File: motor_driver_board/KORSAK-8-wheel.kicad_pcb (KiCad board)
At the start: 2 copper layers, 170 x 90 mm, 20 parts, among them J1 Screw_Terminal_01x04, J2 Conn_01x02_Male, J3 Screw_Terminal_01x06, J4 Screw_Terminal_01x04, M1 Motor_DC, M2 Motor_DC, M3 Motor_DC, M4 Motor_DC, M5 Motor_DC, M6 Motor_DC, M7 Motor_DC, M8 Motor_DC, U1 L293D, U2 L293D, U3 L293D, U4 L293D

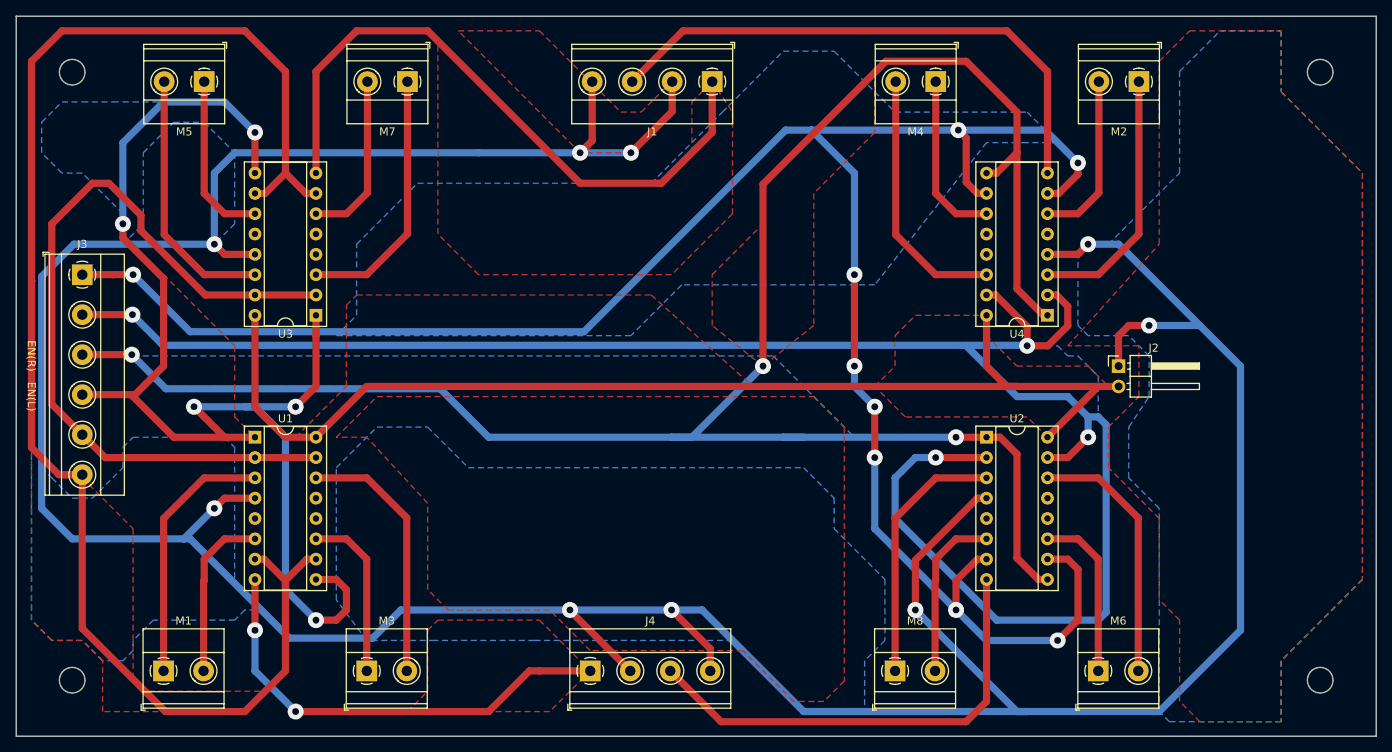
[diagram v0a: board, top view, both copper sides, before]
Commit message: Закончил моделировать плату
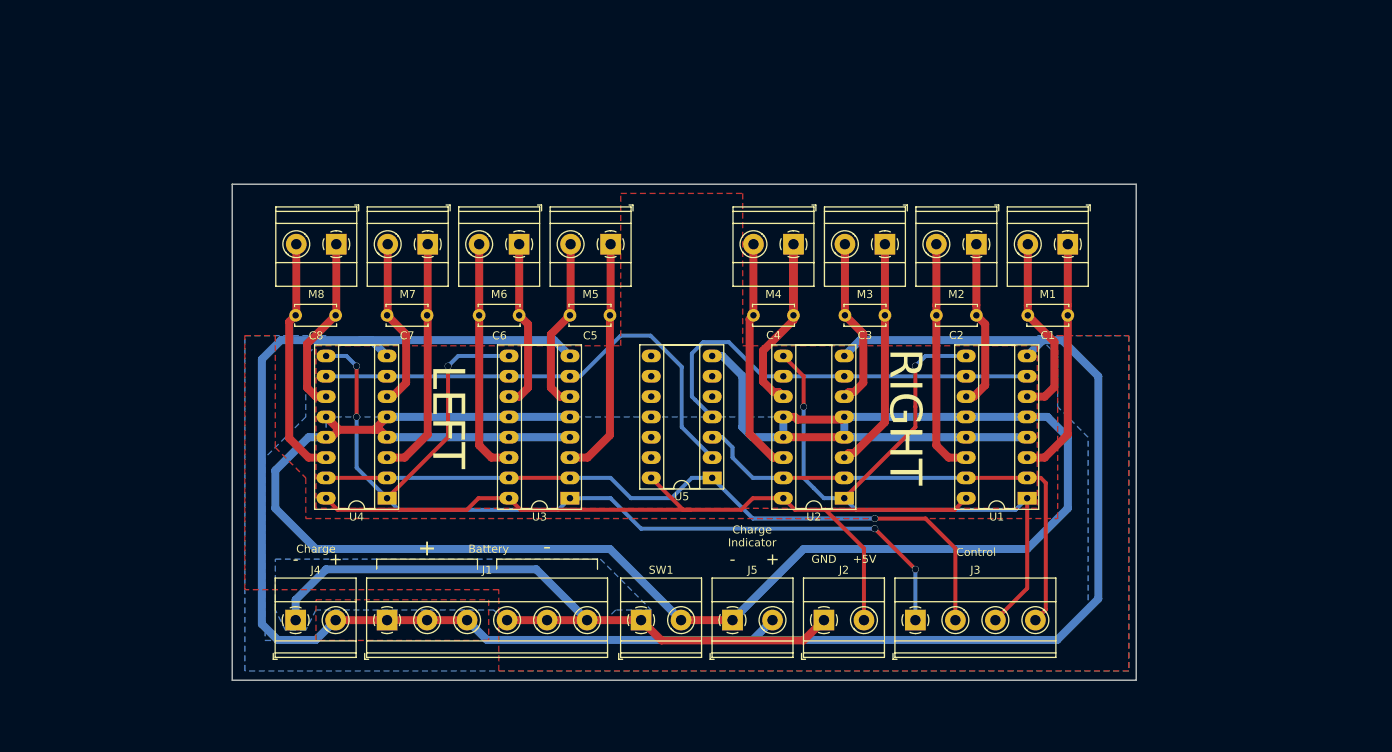
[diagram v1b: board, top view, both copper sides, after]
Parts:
- removed  : MountingHole_3.2mm_M3, MountingHole:MountingHole_3.2mm_M3 (x4)
- added C1: 10pF, Capacitor_THT:C_Disc_D5.0mm_W2.5mm_P5.00mm, F.Cu at (171.4, 72.4)
- added C2: 10pF, Capacitor_THT:C_Disc_D5.0mm_W2.5mm_P5.00mm, F.Cu at (160.0, 72.4)
- added C3: 10pF, Capacitor_THT:C_Disc_D5.0mm_W2.5mm_P5.00mm, F.Cu at (148.6, 72.4)
- added C4: 10pF, Capacitor_THT:C_Disc_D5.0mm_W2.5mm_P5.00mm, F.Cu at (137.2, 72.4)
- added C5: 10pF, Capacitor_THT:C_Disc_D5.0mm_W2.5mm_P5.00mm, F.Cu at (109.2, 72.4)
- added C6: 10pF, Capacitor_THT:C_Disc_D5.0mm_W2.5mm_P5.00mm, F.Cu at (97.9, 72.4)
- added C7: 10pF, Capacitor_THT:C_Disc_D5.0mm_W2.5mm_P5.00mm, F.Cu at (86.4, 72.4)
- added C8: 10pF, Capacitor_THT:C_Disc_D5.0mm_W2.5mm_P5.00mm, F.Cu at (74.9, 72.4)
- added J5: Charge Indicator, TerminalBlock_Phoenix:TerminalBlock_Phoenix_MKDS-1,5-2_1x02_P5.00mm_Horizontal, F.Cu at (129.5, 110.5)
- added SW1: SW_SPST, TerminalBlock_Phoenix:TerminalBlock_Phoenix_MKDS-1,5-2_1x02_P5.00mm_Horizontal, F.Cu at (118.1, 110.5)
- added U5: 74LS04, Package_DIP:DIP-14_W7.62mm_Socket_LongPads, F.Cu at (127.0, 92.7)
- J1: value Screw_Terminal_01x04 -> Battery; footprint TerminalBlock_Phoenix:TerminalBlock_Phoenix_MKDS-1,5-4_1x04_P5.00mm_Horizontal -> TerminalBlock_Phoenix:TerminalBlock_Phoenix_MKDS-1,5-6_1x06_P5.00mm_Horizontal
- J2: value Conn_01x02_Male -> 5V Power; footprint Connector_PinHeader_2.54mm:PinHeader_1x02_P2.54mm_Horizontal -> TerminalBlock_Phoenix:TerminalBlock_Phoenix_MKDS-1,5-2_1x02_P5.00mm_Horizontal
- J3: value Screw_Terminal_01x06 -> Logic Connector; footprint TerminalBlock_Phoenix:TerminalBlock_Phoenix_MKDS-1,5-6_1x06_P5.00mm_Horizontal -> TerminalBlock_Phoenix:TerminalBlock_Phoenix_MKDS-1,5-4_1x04_P5.00mm_Horizontal
- J4: value Screw_Terminal_01x04 -> Charger; footprint TerminalBlock_Phoenix:TerminalBlock_Phoenix_MKDS-1,5-4_1x04_P5.00mm_Horizontal -> TerminalBlock_Phoenix:TerminalBlock_Phoenix_MKDS-1,5-2_1x02_P5.00mm_Horizontal
- U1, U2, U3, U4: footprint Package_DIP:DIP-16_W7.62mm_Socket -> Package_DIP:DIP-16_W7.62mm_Socket_LongPads
- moved M1 125.0 mm to (171.4, 63.5), turned to 180 degrees
- moved J3 112.7 mm to (152.4, 110.5), turned to 0 degrees
- moved U1 96.8 mm to (166.4, 95.2), turned to 180 degrees
- moved M6 89.9 mm to (102.9, 63.5), turned to 180 degrees
- moved M8 87.9 mm to (80.0, 63.5), turned to 180 degrees
- moved U4 85.7 mm to (86.4, 95.2)
- moved M3 83.9 mm to (148.6, 63.5), turned to 180 degrees
- moved J1 78.6 mm to (86.4, 110.5), turned to 0 degrees
- moved M5 54.7 mm to (114.3, 63.5)
- moved J2 48.6 mm to (141.0, 110.5)
- moved U3 39.1 mm to (109.2, 95.2)
- moved J4 37.4 mm to (74.9, 110.5)
- moved M2 28.7 mm to (160.0, 63.5)
- moved M4 27.0 mm to (137.2, 63.5)
- moved M7 20.5 mm to (91.4, 63.5)
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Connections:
- net Net-(M1-Pad1) renamed /M1_OUT_1
- net Net-(M1-Pad2) renamed /M1_OUT_2
- J1 pad 1: Net-(J1-Pad1) -> +BATT
- J1 pad 2: GND -> +BATT
- J1 pad 3: Net-(J1-Pad3) -> +BATT
- J1 pad 4: GND -> /-BATT
- J2 pad 1: GND -> /-BATT
- J3 pad 1: Net-(J3-Pad1) -> /L_EN
- J3 pad 2: Net-(J3-Pad2) -> /L_IN_1
- J3 pad 3: Net-(J3-Pad3) -> /R_EN
- J3 pad 4: Net-(J3-Pad4) -> /R_IN_1
- J4 pad 1: Net-(J4-Pad1) -> /-BATT
- J4 pad 2: GND -> +BATT
- M2 pad 1: Net-(M2-Pad1) -> /M2_OUT_1
- M2 pad 2: Net-(M2-Pad2) -> /M2_OUT_2
- M3 pad 1: Net-(M3-Pad1) -> /M3_OUT_1
- M3 pad 2: Net-(M3-Pad2) -> /M3_OUT_2
- M4 pad 1: Net-(M4-Pad1) -> /M4_OUT_1
- M4 pad 2: Net-(M4-Pad2) -> /M4_OUT_2
- M5 pad 1: Net-(M5-Pad1) -> /M6_OUT_1
- M5 pad 2: Net-(M5-Pad2) -> /M6_OUT_2
- M6 pad 1: Net-(M6-Pad1) -> /M5_OUT_1
- M6 pad 2: Net-(M6-Pad2) -> /M5_OUT_2
- M7 pad 1: Net-(M7-Pad1) -> /M8_OUT_1
- M7 pad 2: Net-(M7-Pad2) -> /M8_OUT_2
- M8 pad 1: Net-(M8-Pad1) -> /M7_OUT_1
- M8 pad 2: Net-(M8-Pad2) -> /M7_OUT_2
- U1 pad 1: Net-(J3-Pad4) -> /R_EN
- U1 pad 10: Net-(J3-Pad6) -> /R_IN_2
- U1 pad 11: Net-(M3-Pad1) -> /M2_OUT_1
- U1 pad 14: Net-(M3-Pad2) -> /M2_OUT_2
- U1 pad 15: Net-(J3-Pad5) -> /R_IN_1
- U1 pad 2: Net-(J3-Pad5) -> /R_IN_1
- U1 pad 7: Net-(J3-Pad6) -> /R_IN_2
- U1 pad 8: Net-(J4-Pad1) -> +BATT
- U1 pad 9: Net-(J3-Pad4) -> /R_EN
- U2 pad 1: Net-(J3-Pad3) -> /R_EN
- U2 pad 10: Net-(J3-Pad1) -> /R_IN_2
- U2 pad 11: Net-(M6-Pad1) -> /M4_OUT_1
- U2 pad 14: Net-(M6-Pad2) -> /M4_OUT_2
- U2 pad 15: Net-(J3-Pad2) -> /R_IN_1
- U2 pad 2: Net-(J3-Pad2) -> /R_IN_1
- U2 pad 3: Net-(M8-Pad1) -> /M3_OUT_1
- U2 pad 6: Net-(M8-Pad2) -> /M3_OUT_2
- U2 pad 7: Net-(J3-Pad1) -> /R_IN_2
- U2 pad 8: Net-(J4-Pad3) -> +BATT
- U2 pad 9: Net-(J3-Pad3) -> /R_EN
- U3 pad 1: Net-(J3-Pad4) -> /L_EN
- U3 pad 10: Net-(J3-Pad6) -> /L_IN_2
- U3 pad 11: Net-(M5-Pad1) -> /M5_OUT_1
- U3 pad 14: Net-(M5-Pad2) -> /M5_OUT_2
- U3 pad 15: Net-(J3-Pad5) -> /L_IN_1
- U3 pad 2: Net-(J3-Pad5) -> /L_IN_1
- U3 pad 3: Net-(M7-Pad1) -> /M6_OUT_1
- U3 pad 6: Net-(M7-Pad2) -> /M6_OUT_2
- U3 pad 7: Net-(J3-Pad6) -> /L_IN_2
- U3 pad 8: Net-(J1-Pad1) -> +BATT
- U3 pad 9: Net-(J3-Pad4) -> /L_EN
- U4 pad 1: Net-(J3-Pad3) -> /L_EN
- U4 pad 10: Net-(J3-Pad1) -> /L_IN_2
- U4 pad 11: Net-(M4-Pad1) -> /M7_OUT_1
- U4 pad 14: Net-(M4-Pad2) -> /M7_OUT_2
- U4 pad 15: Net-(J3-Pad2) -> /L_IN_1
- U4 pad 2: Net-(J3-Pad2) -> /L_IN_1
- U4 pad 3: Net-(M2-Pad1) -> /M8_OUT_1
- U4 pad 6: Net-(M2-Pad2) -> /M8_OUT_2
- U4 pad 7: Net-(J3-Pad1) -> /L_IN_2
- U4 pad 8: Net-(J1-Pad3) -> +BATT
- U4 pad 9: Net-(J3-Pad3) -> /L_EN
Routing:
- net Net-(J3-Pad1): track 260.4 -> 0.00 mm, vias 9 -> 0
- net +BATT: track 0.00 -> 255.6 mm
- net Net-(J3-Pad3): track 253.2 -> 0.00 mm, vias 3 -> 0
- net Net-(J3-Pad2): track 243.9 -> 0.00 mm, vias 4 -> 0
- net Net-(J3-Pad6): track 186.0 -> 0.00 mm
- net GND: track 455.3 -> 280.3 mm, vias 9 -> 0
- net Net-(J3-Pad4): track 157.5 -> 0.00 mm, vias 5 -> 0
- net /L_EN: track 0.00 -> 127.5 mm, vias 0 -> 5
- net Net-(J3-Pad5): track 100.4 -> 0.00 mm
- net /L_IN_1: track 0.00 -> 94.4 mm, vias 0 -> 1
- net /R_EN: track 0.00 -> 90.4 mm, vias 0 -> 2
- net /-BATT: track 0.00 -> 84.9 mm
- net Net-(J1-Pad1): track 81.2 -> 0.00 mm
- net Net-(J1-Pad3): track 69.3 -> 0.00 mm
- net /R_IN_1: track 0.00 -> 62.5 mm
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- added copper zone on B.Cu, net +BATT
- added copper zone on F.Cu, net +BATT
- added copper zone on B.Cu, net /-BATT
- added copper zone on F.Cu, net /-BATT
- removed copper zone on F.Cu, net +5V
- removed copper zone on F.Cu, net Net-(J1-Pad1)
- removed copper zone on B.Cu, net Net-(J3-Pad1)
- removed copper zone on B.Cu, net Net-(J3-Pad2)
- removed copper zone on B.Cu, net Net-(J3-Pad3)
- removed copper zone on F.Cu, net Net-(J3-Pad3)
- removed copper zone on B.Cu, net Net-(J3-Pad4)
- removed copper zone on F.Cu, net Net-(J3-Pad4)
- removed copper zone on F.Cu, net Net-(J3-Pad6)
- removed copper zone on F.Cu, net Net-(J4-Pad1)
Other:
- board size 170 x 90 mm -> 113 x 62 mm
- net class 5V (logic) added: clearance 0.4, trace_width 0.5, via_dia 0.85, via_drill 0.8
- net class Default: clearance 0.8 -> 0.4; trace_width 0.9 -> 0.3; via_dia 2 -> 0.85; via_drill 0.85 -> 0.8
- net class power added: clearance 0.68, trace_width 1, via_dia 0.85, via_drill 0.8
- rule trace_clearance: 0.8 -> 0.4
- board text added: "+"
- board text added: "+5V"
- board text added: "-"
- board text added: "Battery"
- board text added: "Charge"
- board text added: "Charge Indicator"
- board text added: "Control"
- board text added: "GND"
- board text added: "LEFT"
- board text added: "RIGHT"
- board text removed: "EN(L)"
- board text removed: "EN(R)"
